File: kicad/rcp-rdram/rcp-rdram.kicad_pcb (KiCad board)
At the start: 2 copper layers, 36.8 x 54.6 mm, 29 parts, among them P1 RDRAM-EDGE, U11 RDRAM18-NUS, U11-2 RDRAM18-NUS, U14 RDRAM18-NUS, U14-2 RDRAM18-NUS, U15 MX8330, X2 14.705MHz

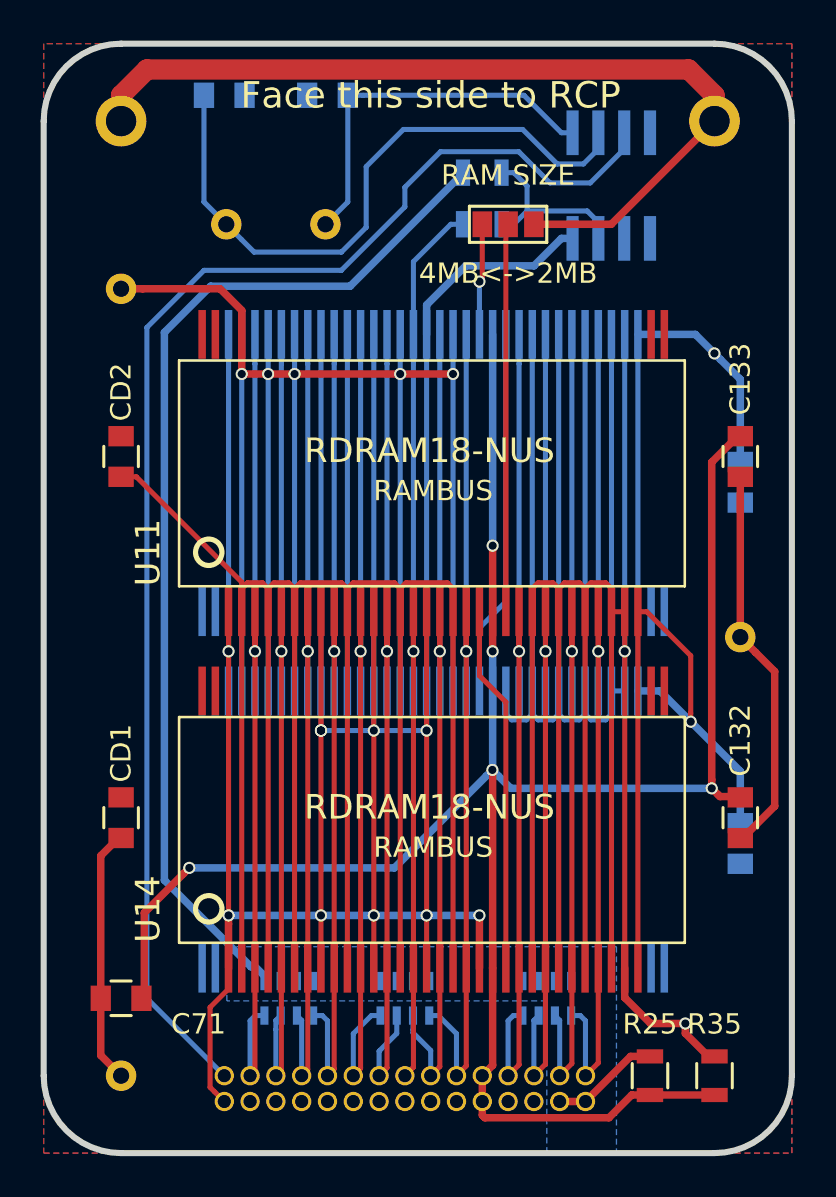
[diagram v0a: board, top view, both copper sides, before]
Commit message: Completed, DRC check pass
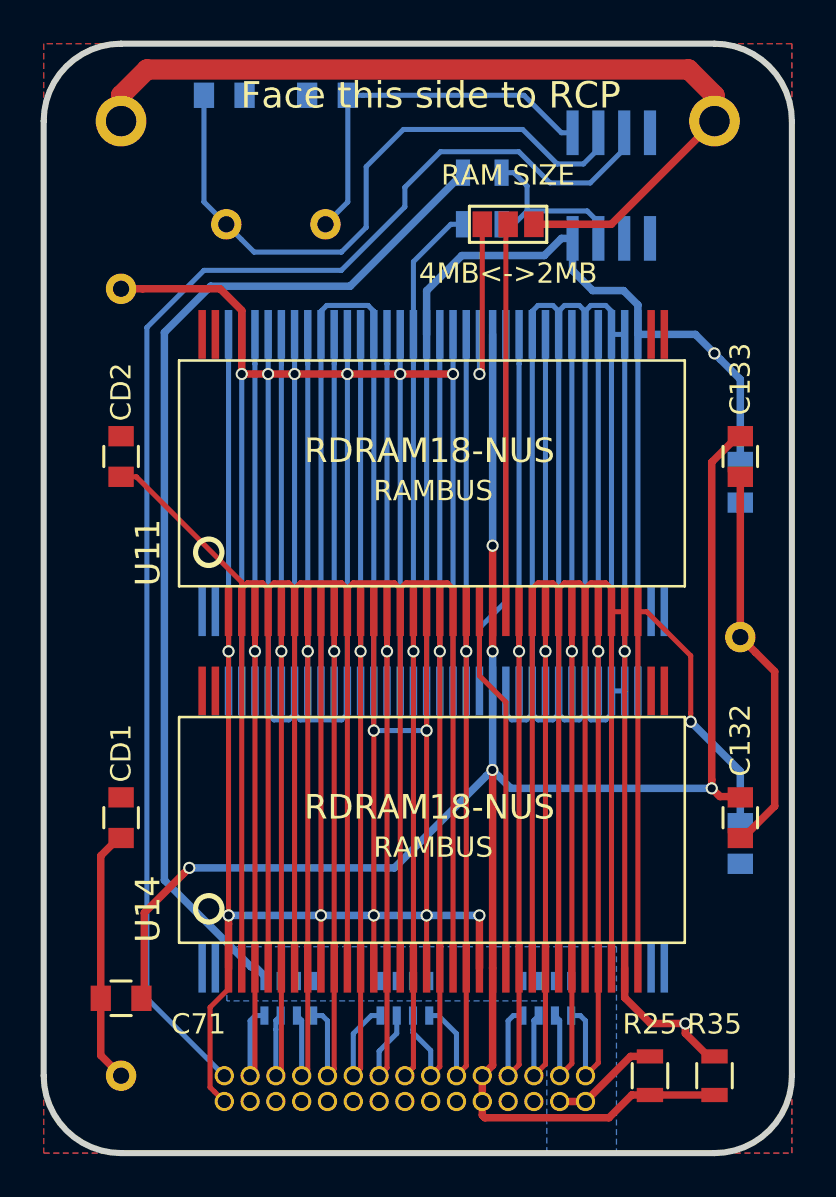
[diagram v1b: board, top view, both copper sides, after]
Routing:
- net GND: track 539.3 -> 556.9 mm, vias 7 -> 8
- net VDD: track 249.3 -> 254.0 mm, vias 12 -> 10
- net Net-(JP1-Pad1): track 5.48 -> 9.38 mm
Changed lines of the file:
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@@
   (general
     (links 199)
-    (no_connects 59)
+    (no_connects 3)
     (area 101.449999 76.049999 138.580001 130.960001)
     (thickness 1.6)
     (drawings 13)
-    (tracks 444)
+    (tracks 475)
     (zones 0)
     (modules 29)
@@
   (segment (start 129.424999 129.070001) (end 130.545 127.95) (width 0.37) (layer F.Cu) (net 1))
   (segment (start 130.545 127.95) (end 131.445 127.95) (width 0.37) (layer F.Cu) (net 1))
+  (segment (start 113.949999 108.059999) (end 113.949999 109.200001) (width 0.25) (layer B.Cu) (net 2))
+  (segment (start 113.949999 109.200001) (end 114.234998 109.485) (width 0.25) (layer B.Cu) (net 2))
+  (segment (start 114.234998 109.485) (end 116.265 109.485) (width 0.25) (layer B.Cu) (net 2))
+  (segment (start 116.265 109.485) (end 116.549999 109.200001) (width 0.25) (layer B.Cu) (net 2))
+  (segment (start 116.549999 109.200001) (end 116.549999 108.059999) (width 0.25) (layer B.Cu) (net 2))
+  (segment (start 113.949999 109.200001) (end 113.665 109.485) (width 0.25) (layer B.Cu) (net 2))
+  (segment (start 113.665 109.485) (end 112.934998 109.485) (width 0.25) (layer B.Cu) (net 2))
+  (segment (start 112.934998 109.485) (end 112.649999 109.200001) (width 0.25) (layer B.Cu) (net 2))
+  (segment (start 112.649999 109.200001) (end 112.649999 108.059999) (width 0.25) (layer B.Cu) (net 2))
+  (segment (start 129.55 90.51) (end 130.2 90.51) (width 0.25) (layer B.Cu) (net 2))
+  (segment (start 128.25 90.51) (end 128.25 89.369998) (width 0.25) (layer B.Cu) (net 2))
+  (segment (start 128.25 89.369998) (end 128.534999 89.084999) (width 0.25) (layer B.Cu) (net 2))
+  (segment (start 128.534999 89.084999) (end 129.265001 89.084999) (width 0.25) (layer B.Cu) (net 2))
+  (segment (start 129.265001 89.084999) (end 129.55 89.369998) (width 0.25) (layer B.Cu) (net 2))
+  (segment (start 129.55 89.369998) (end 129.55 90.51) (width 0.25) (layer B.Cu) (net 2))
+  (segment (start 126.95 90.51) (end 126.95 89.369998) (width 0.25) (layer B.Cu) (net 2))
+  (segment (start 126.95 89.369998) (end 127.234999 89.084999) (width 0.25) (layer B.Cu) (net 2))
+  (segment (start 127.234999 89.084999) (end 127.965001 89.084999) (width 0.25) (layer B.Cu) (net 2))
+  (segment (start 127.965001 89.084999) (end 128.25 89.369998) (width 0.25) (layer B.Cu) (net 2))
+  (segment (start 125.65 90.51) (end 125.65 89.369998) (width 0.25) (layer B.Cu) (net 2))
+  (segment (start 125.65 89.369998) (end 125.934999 89.084999) (width 0.25) (layer B.Cu) (net 2))
+  (segment (start 125.934999 89.084999) (end 126.665001 89.084999) (width 0.25) (layer B.Cu) (net 2))
+  (segment (start 126.665001 89.084999) (end 126.95 89.369998) (width 0.25) (layer B.Cu) (net 2))
+  (segment (start 116.549999 92.46) (end 116.549999 108.059999) (width 0.25) (layer B.Cu) (net 2))
+  (segment (start 116.549999 90.51) (end 116.549999 92.46) (width 0.25) (layer B.Cu) (net 2))
+  (via (at 116.549999 92.46) (size 0.6) (drill 0.4) (layers F.Cu B.Cu) (net 2))
   (segment (start 121.75 92.46) (end 119.149999 92.46) (width 0.37) (layer F.Cu) (net 2))
   (segment (start 121.75 92.46) (end 121.75 108.059999) (width 0.25) (layer B.Cu) (net 2))
@@
   (segment (start 104.41 123.19) (end 104.41 126) (width 0.37) (layer F.Cu) (net 2))
   (segment (start 104.41 126) (end 105.41 127) (width 0.37) (layer F.Cu) (net 2))
-  (segment (start 116.549999 90.51) (end 116.549999 108.059999) (width 0.25) (layer B.Cu) (net 2))
   (segment (start 125.65 108.059999) (end 125.65 90.51) (width 0.25) (layer B.Cu) (net 2))
   (segment (start 126.95 108.059999) (end 126.95 90.51) (width 0.25) (layer B.Cu) (net 2))
@@
   (segment (start 116.57 78.74) (end 116.57 83.99094) (width 0.25) (layer B.Cu) (net 4))
   (segment (start 116.57 83.99094) (end 115.47094 85.09) (width 0.25) (layer B.Cu) (net 4))
-  (segment (start 115.25 110.01) (end 117.85 110.01) (width 0.25) (layer B.Cu) (net 5))
-  (segment (start 117.85 110.01) (end 120.449999 110.01) (width 0.25) (layer B.Cu) (net 5))
+  (segment (start 130.85 90.51) (end 130.85 89.06) (width 0.37) (layer B.Cu) (net 5))
+  (segment (start 128.622969 88.353831) (end 127.635062 87.365924) (width 0.37) (layer B.Cu) (net 5))
+  (segment (start 130.143831 88.353831) (end 128.622969 88.353831) (width 0.37) (layer B.Cu) (net 5))
+  (segment (start 130.85 89.06) (end 130.143831 88.353831) (width 0.37) (layer B.Cu) (net 5))
+  (segment (start 127.635062 87.365924) (end 127.635062 85.785063) (width 0.37) (layer B.Cu) (net 5))
+  (segment (start 120.449999 90.51) (end 120.449999 88.360947) (width 0.37) (layer B.Cu) (net 5))
+  (segment (start 120.449999 88.360947) (end 122.181988 86.628958) (width 0.37) (layer B.Cu) (net 5))
+  (segment (start 127.085062 85.785063) (end 127.635062 85.785063) (width 0.37) (layer B.Cu) (net 5))
+  (segment (start 122.181988 86.628958) (end 126.241167 86.628958) (width 0.37) (layer B.Cu) (net 5))
+  (segment (start 126.241167 86.628958) (end 127.085062 85.785063) (width 0.37) (layer B.Cu) (net 5))
+  (segment (start 120.449999 110.01) (end 117.85 110.01) (width 0.25) (layer B.Cu) (net 5))
+  (segment (start 120.449999 119.11) (end 123.05 119.11) (width 0.37) (layer B.Cu) (net 5))
+  (segment (start 117.849999 119.11) (end 120.449999 119.11) (width 0.37) (layer B.Cu) (net 5))
+  (segment (start 115.249999 119.11) (end 117.849999 119.11) (width 0.37) (layer B.Cu) (net 5))
+  (segment (start 110.7 119.11) (end 115.249999 119.11) (width 0.37) (layer B.Cu) (net 5))
+  (segment (start 115.249999 90.51) (end 115.249999 89.369998) (width 0.25) (layer B.Cu) (net 5))
+  (segment (start 115.249999 89.369998) (end 115.534998 89.084999) (width 0.25) (layer B.Cu) (net 5))
+  (segment (start 115.534998 89.084999) (end 117.565 89.084999) (width 0.25) (layer B.Cu) (net 5))
+  (segment (start 117.565 89.084999) (end 117.849999 89.369998) (width 0.25) (layer B.Cu) (net 5))
+  (segment (start 117.849999 89.369998) (end 117.849999 90.51) (width 0.25) (layer B.Cu) (net 5))
   (segment (start 117.849999 108.059999) (end 117.849999 110.009999) (width 0.25) (layer B.Cu) (net 5))
   (segment (start 117.849999 110.009999) (end 117.85 110.01) (width 0.25) (layer B.Cu) (net 5))
   (via (at 117.85 110.01) (size 0.6) (drill 0.4) (layers F.Cu B.Cu) (net 5))
-  (via (at 115.25 110.01) (size 0.6) (drill 0.4) (layers F.Cu B.Cu) (net 5))
-  (segment (start 115.249999 108.059999) (end 115.249999 110.009999) (width 0.25) (layer B.Cu) (net 5))
-  (segment (start 115.249999 110.009999) (end 115.25 110.01) (width 0.25) (layer B.Cu) (net 5))
-  (via (at 115.25 110.01) (size 0.6) (drill 0.4) (layers F.Cu B.Cu) (net 5))
   (segment (start 120.449999 108.059999) (end 120.449999 110.01) (width 0.25) (layer B.Cu) (net 5))
   (segment (start 120.449999 108.06) (end 120.449999 104.16) (width 0.25) (layer F.Cu) (net 5))
@@
   (segment (start 120.449999 108.06) (end 120.449999 110.01) (width 0.25) (layer F.Cu) (net 5))
   (via (at 120.449999 110.01) (size 0.6) (drill 0.4) (layers F.Cu B.Cu) (net 5))
-  (segment (start 123.05 119.11) (end 110.7 119.11) (width 0.37) (layer B.Cu) (net 5))
   (segment (start 120.449999 90.51) (end 120.449999 108.059999) (width 0.25) (layer B.Cu) (net 5))
   (segment (start 130.85 104.16) (end 131.285 104.16) (width 0.25) (layer F.Cu) (net 5))
@@
   (segment (start 133.45 106.325) (end 133.45 109.150076) (width 0.25) (layer F.Cu) (net 5))
   (segment (start 133.45 109.150076) (end 133.45 109.57434) (width 0.25) (layer F.Cu) (net 5))
-  (segment (start 133.45 109.57434) (end 131.935659 108.059999) (width 0.37) (layer B.Cu) (net 5))
   (segment (start 135.89 112.01434) (end 133.45 109.57434) (width 0.37) (layer B.Cu) (net 5))
   (via (at 133.45 109.57434) (size 0.6) (drill 0.4) (layers F.Cu B.Cu) (net 5))
@@
   (via (at 110.699999 106.11) (size 0.6) (drill 0.4) (layers F.Cu B.Cu) (net 5))
   (segment (start 135.89 114.57) (end 135.89 112.01434) (width 0.37) (layer B.Cu) (net 5))
-  (segment (start 131.935659 108.059999) (end 130.85 108.059999) (width 0.37) (layer B.Cu) (net 5))
-  (segment (start 120.449999 90.51) (end 120.449999 89.06) (width 0.37) (layer B.Cu) (net 5))
-  (segment (start 127.085062 85.785063) (end 127.635062 85.785063) (width 0.37) (layer B.Cu) (net 5))
-  (segment (start 125.735062 87.135063) (end 127.085062 85.785063) (width 0.37) (layer B.Cu) (net 5))
-  (segment (start 122.374936 87.135063) (end 125.735062 87.135063) (width 0.37) (layer B.Cu) (net 5))
-  (segment (start 120.449999 89.06) (end 122.374936 87.135063) (width 0.37) (layer B.Cu) (net 5))
   (segment (start 134.615788 91.44606) (end 133.679728 90.51) (width 0.37) (layer B.Cu) (net 5))
   (via (at 134.615788 91.44606) (size 0.6) (drill 0.4) (layers F.Cu B.Cu) (net 5))
@@
   (segment (start 124.35 103.65915) (end 124.35 90.51) (width 0.25) (layer B.Cu) (net 24))
   (segment (start 123.05 108.059999) (end 123.05 104.95915) (width 0.25) (layer B.Cu) (net 24))
-  (segment (start 123.19 87.77) (end 123.05 87.91) (width 0.25) (layer F.Cu) (net 27))
-  (segment (start 123.19 85.09) (end 123.19 87.77) (width 0.25) (layer F.Cu) (net 27))
-  (segment (start 123.05 87.91) (end 123.05 90.51) (width 0.25) (layer B.Cu) (net 27))
-  (via (at 123.05 87.91) (size 0.6) (drill 0.4) (layers F.Cu B.Cu) (net 27))
+  (segment (start 123.05 92.46) (end 123.05 90.51) (width 0.25) (layer B.Cu) (net 27))
+  (segment (start 123.19 85.09) (end 123.19 92.32) (width 0.25) (layer F.Cu) (net 27))
+  (segment (start 123.19 92.32) (end 123.05 92.46) (width 0.25) (layer F.Cu) (net 27))
+  (via (at 123.05 92.46) (size 0.6) (drill 0.4) (layers F.Cu B.Cu) (net 27))
   (zone (net 2) (net_name GND) (layer B.Cu) (hatch edge 0.508)
     (connect_pads (clearance 0.508))
